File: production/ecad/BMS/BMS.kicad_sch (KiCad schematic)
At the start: 11 parts, among them J11 2147210040, J7 ADC-028-1-T/R-PA10T, U4 TPS75233QPWPREP

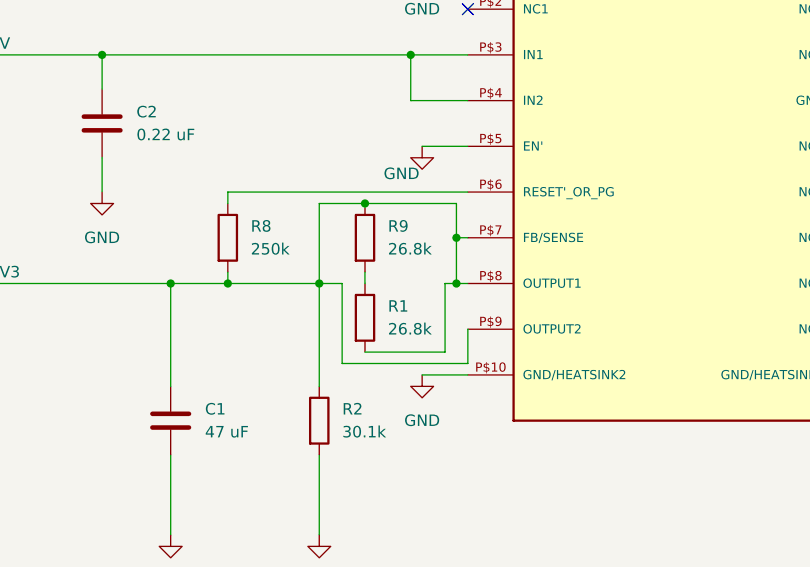
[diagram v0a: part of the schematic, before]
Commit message: some changes
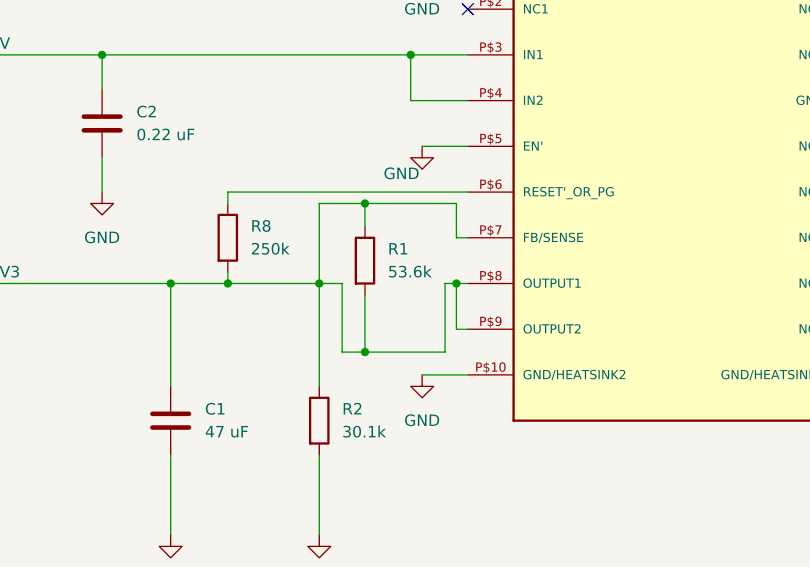
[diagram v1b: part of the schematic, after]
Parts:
- removed R1: 26.8k, Resistor_SMD:R_0201_0603Metric, symbol Device:R
- C1: footprint Capacitor_SMD:C_0603_1608Metric -> Capacitor_SMD:C_0805_2012Metric
- R1: renamed from R9; value 26.8k -> 53.6k; footprint Resistor_SMD:R_0201_0603Metric -> Resistor_SMD:R_0805_2012Metric
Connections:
- net +3V3: now also R1.2
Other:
- moved on the sheet: R1
